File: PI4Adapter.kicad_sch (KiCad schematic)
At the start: 5 parts, among them J1 Conn_02x20_Odd_Even, J2 Conn_02x20_Odd_Even, J3 Conn_02x13_Odd_Even, J4 Conn_01x02_Male, U1 USB_C_2.0

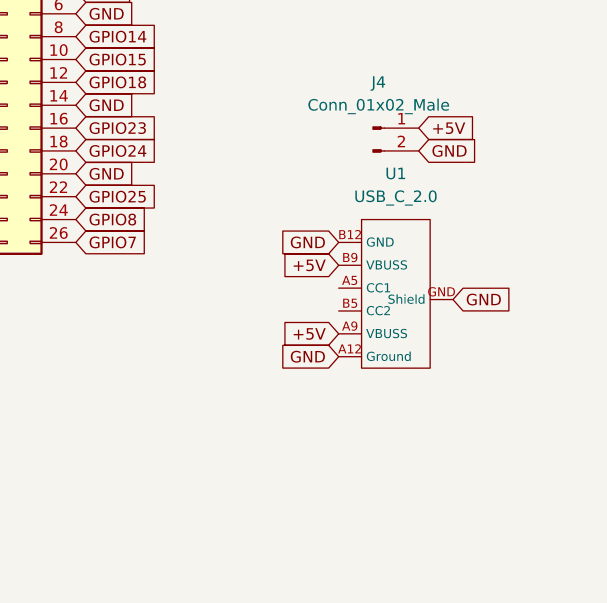
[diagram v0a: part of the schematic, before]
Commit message: update
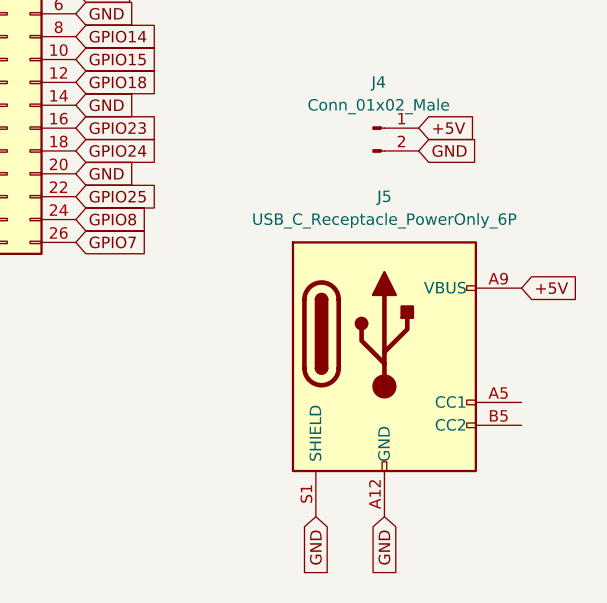
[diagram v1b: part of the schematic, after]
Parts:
- removed U1: USB_C_2.0, Library:USB_C_C31M17, symbol PI4Adapter:USB_C_2.0
- added J5: USB_C_Receptacle_PowerOnly_6P, Connector_USB:USB_C_Receptacle_GCT_USB4135-GF-A_6P_TopMnt_Horizontal, symbol Connector:USB_C_Receptacle_PowerOnly_6P
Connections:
- net +5V: now also J5.A9 (VBUS), J5.B9 (VBUS)
- net GND: now also J5.A12 (GND), J5.B12 (GND), J5.S1 (SHIELD)
